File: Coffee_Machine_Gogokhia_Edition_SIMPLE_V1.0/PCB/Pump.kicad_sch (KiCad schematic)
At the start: 8 parts, among them J12 PUMP_TAB, Q5 BT131, U8 MOC3021M

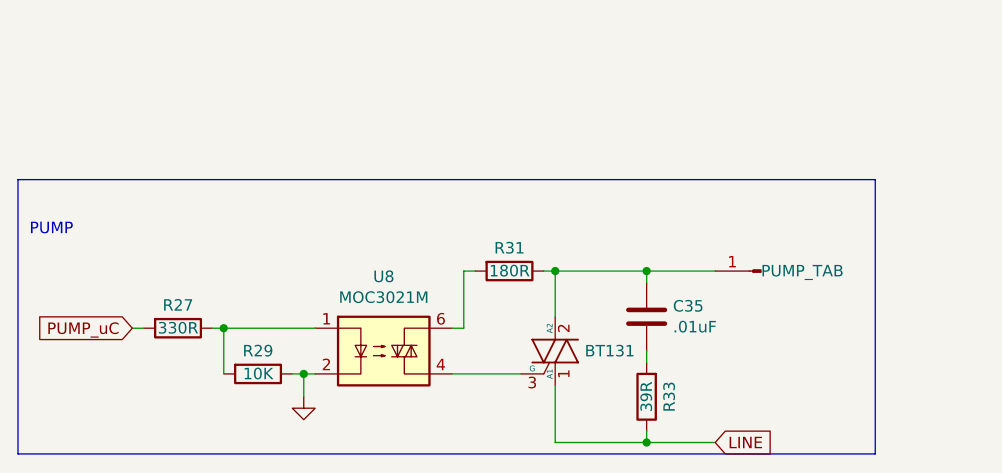
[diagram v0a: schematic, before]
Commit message: 1
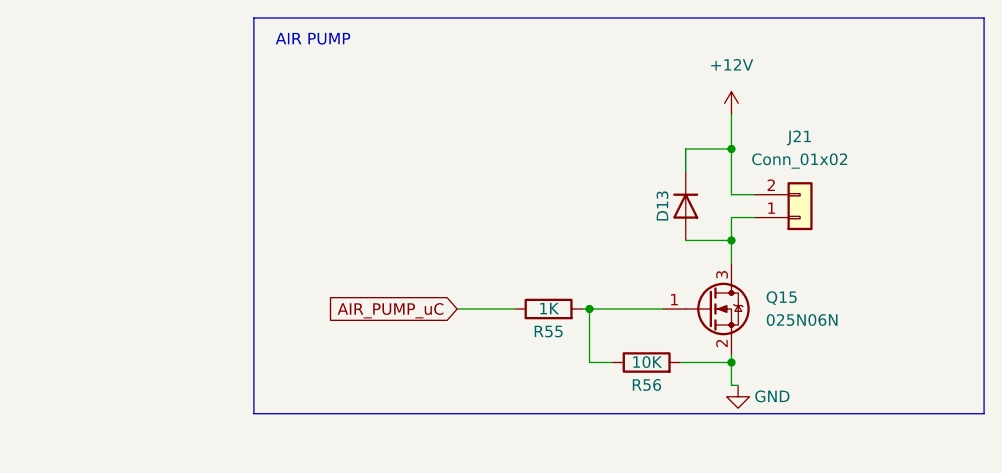
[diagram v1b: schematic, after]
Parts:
- removed C35: .01uF, Capacitor_THT:C_Disc_D5.0mm_W2.5mm_P5.00mm, symbol Device:C
- removed J12: PUMP_TAB, Footprint:TAB_Conn, symbol Connector:Conn_01x01_Male
- removed Q5: BT131, Footprint:BT131, symbol Triac_Thyristor:BTA16-600B
- removed R27: 330R, Resistor_SMD:R_0603_1608Metric, symbol Device:R
- removed R29: 10K, Resistor_SMD:R_0603_1608Metric, symbol Device:R
- removed R31: 180R, Resistor_SMD:R_1206_3216Metric, symbol Device:R
- removed R33: 39R, Resistor_SMD:R_1206_3216Metric, symbol Device:R
- removed U8: MOC3021M, Footprint:DIP6_SMD, symbol Relay_SolidState:MOC3021M
- added D13: D, Diode_SMD:D_SMA, symbol Device:D
- added J21: Conn_01x02, Footprint:JST_2.54_2P, symbol Connector_Generic:Conn_01x02
- added Q15: 025N06N, Package_TO_SOT_SMD:TO-252-2, symbol Transistor_FET:AO3400A
- added R55: 1K, Resistor_SMD:R_0603_1608Metric, symbol Device:R
- added R56: 10K, Resistor_SMD:R_0603_1608Metric, symbol Device:R
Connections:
- net GND: now also Q15.2 (S), R56.2
- new net: D13.2 (A), J21.1 (Pin_1), Q15.3 (D)
- new net: Q15.1 (G), R55.2, R56.1
- new net +12V: D13.1 (K), J21.2 (Pin_2)
- new net AIR_PUMP_uC: R55.1
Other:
- note added: "AIR PUMP"
- note removed: "PUMP"
